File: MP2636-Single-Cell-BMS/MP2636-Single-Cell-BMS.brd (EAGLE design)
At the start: 87.6 x 100 mm, 58 parts, among them U1 MP2636GR-P

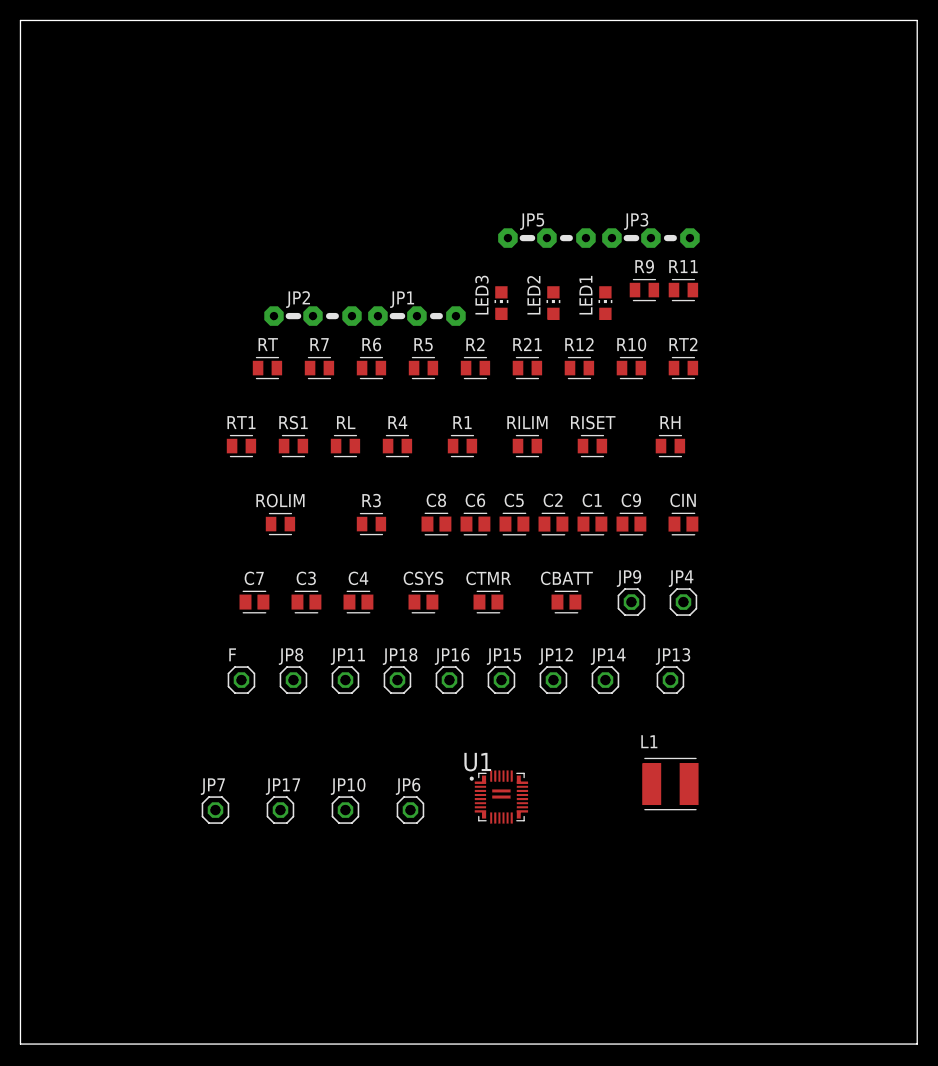
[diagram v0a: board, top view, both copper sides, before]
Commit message: Tentative component placements
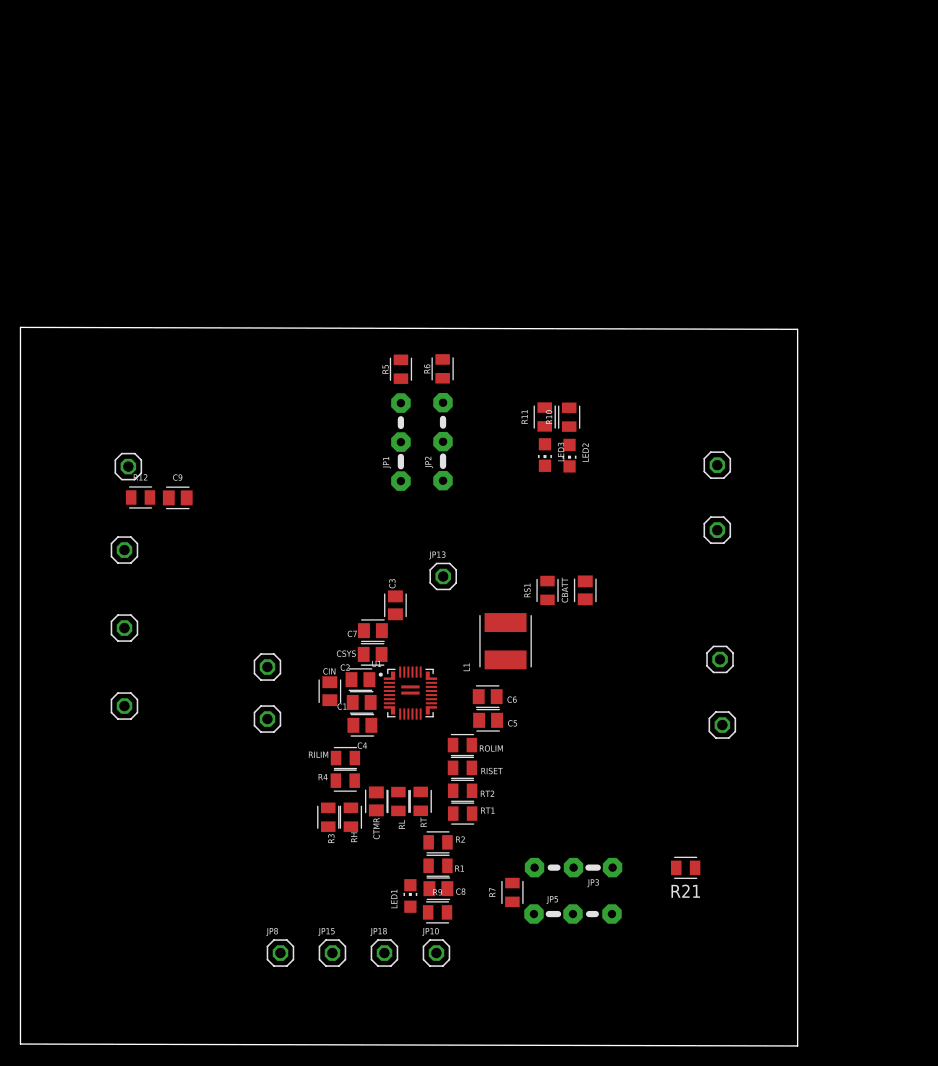
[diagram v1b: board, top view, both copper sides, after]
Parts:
- moved JP5 66.1 mm to (52.1, 12.7)
- moved R9 64.1 mm to (40.8, 12.9)
- moved JP3 61.6 mm to (55.9, 17.2), turned to 180 degrees
- moved LED1 61.0 mm to (38.1, 14.5)
- moved R7 54.6 mm to (48.1, 14.8), turned to 90 degrees
- moved R21 51.2 mm to (65.0, 17.2), turned to 180 degrees
- moved JP9 50.6 mm to (10.2, 33.0)
- moved JP7 50.2 mm to (68.6, 31.2)
- moved RH 47.8 mm to (32.3, 22.2), turned to 270 degrees
- moved RT2 46.6 mm to (43.2, 24.7), turned to 180 degrees
- moved R2 46.5 mm to (40.8, 19.7)
- moved JP12 46.5 mm to (10.5, 56.4)
- moved RT 44.9 mm to (39.1, 23.7), turned to 270 degrees
- moved R12 44.7 mm to (11.7, 53.4)
- moved C9 44.4 mm to (15.4, 53.4)
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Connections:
- net AGND: now also JP1.1, JP2.1, JP3.1, U1.26
- net DGND: no longer JP1.1, JP2.1, JP3.1, U1.26
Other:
- board size 87.6 x 100 mm -> 75.9 x 70.2 mm
